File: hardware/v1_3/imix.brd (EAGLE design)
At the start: 87 x 102.5 mm, 154 parts, among them J2_3_5_AND_6 ARDUINO_R3NO_HOLES, U1 BQ2423X, U10 ISL29035, U11 FX0S8700CQ, U12 296-12686-1-ND, U13 SIP32401A, U14 SIP32401A, U15 SIP32401A, U16 SIP32401A, U17 74LVC4066BQ, U18 74LVC4066BQ, U3 TLV3202, U4 LM358, U5 LDO-TPS78233, U6 ATSAM4LCX_100, U8 SI7021, U9 NRF51422, X1 16MHz, X2 16MHz, X3 16MHz

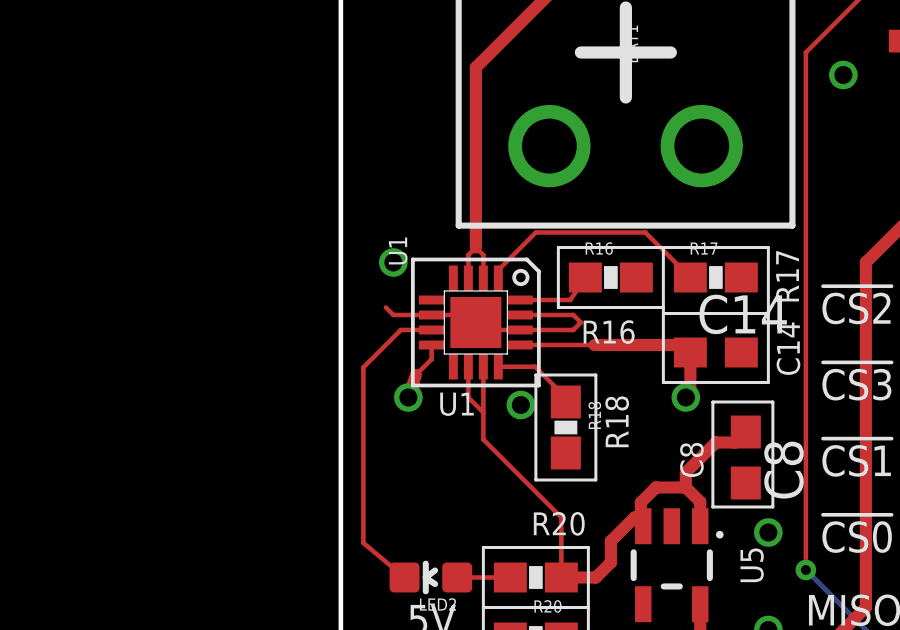
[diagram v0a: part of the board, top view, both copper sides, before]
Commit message: Create PDF
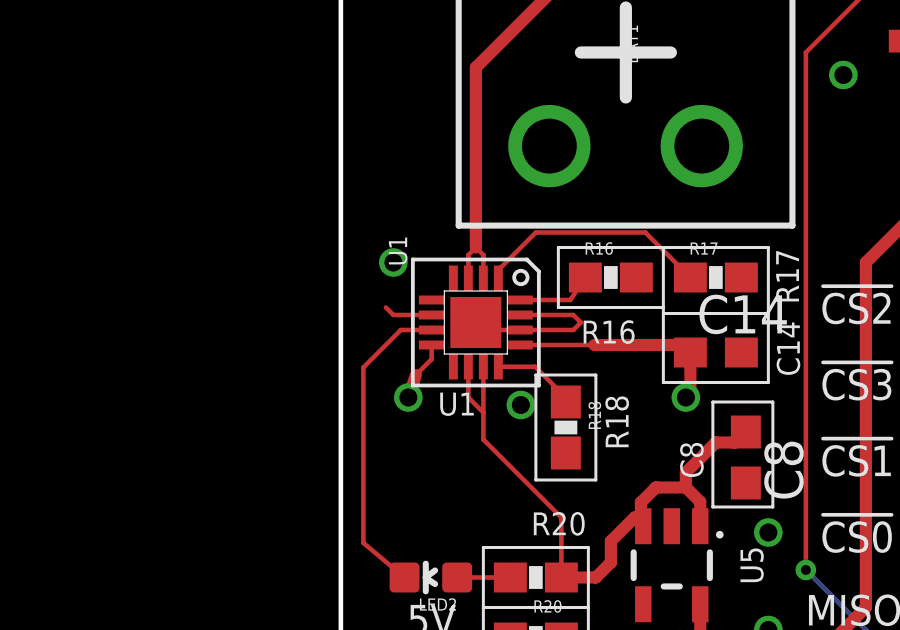
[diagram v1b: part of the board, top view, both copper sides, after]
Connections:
- net GND: no longer U1.6
- net VCC_IN: now also U1.6
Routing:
- net GND: track 215.8 -> 213.0 mm
- net VCC_IN: track 83.9 -> 85.5 mm
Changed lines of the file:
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@@
 <contactref element="R16" pad="2"/>
 <contactref element="U1" pad="4"/>
-<contactref element="U1" pad="6"/>
 <contactref element="U1" pad="5"/>
 <contactref element="U1" pad="14"/>
@@
 <wire x1="50.747" y1="69.824" x2="50.747" y2="67.247" width="0.1524" layer="1"/>
 <wire x1="50.747" y1="67.247" x2="50.5355" y2="67.0355" width="0.1524" layer="1"/>
-<wire x1="3.025" y1="53.25" x2="4.25" y2="53.25" width="0.1524" layer="1"/>
 <wire x1="4.25" y1="53.25" x2="4.5" y2="53" width="0.1524" layer="1"/>
 <via x="43" y="17.5" extent="1-16" drill="0.3302"/>
@@
 <wire x1="77.5" y1="-3.6" x2="79.65" y2="-3.6" width="0.1524" layer="1"/>
 <wire x1="3" y1="53.775" x2="3.025" y2="53.75" width="0.1524" layer="1"/>
-<wire x1="3.025" y1="53.25" x2="1.75" y2="53.25" width="0.1524" layer="1"/>
-<wire x1="1.75" y1="53.25" x2="1.5" y2="53.5" width="0.1524" layer="1"/>
 <wire x1="3.025" y1="52.25" x2="3.025" y2="51.775" width="0.1524" layer="1"/>
 <wire x1="3.025" y1="51.775" x2="2.5" y2="51.25" width="0.1524" layer="1"/>
@@
 <wire x1="6" y1="50.25" x2="7.5" y2="48.65" width="0" layer="19" extent="1-1"/>
 <wire x1="5.975" y1="52.75" x2="6" y2="50.25" width="0" layer="19" extent="1-1"/>
-<wire x1="3.025" y1="53.75" x2="3.025" y2="53.25" width="0" layer="19" extent="1-1"/>
-<wire x1="3.025" y1="52.25" x2="3.025" y2="53.25" width="0" layer="19" extent="1-1"/>
-<wire x1="3.75" y1="54.475" x2="3.025" y2="53.75" width="0" layer="19" extent="1-1"/>
-<wire x1="1.75" y1="55" x2="1.5" y2="53.5" width="0" layer="19" extent="1-1"/>
+<wire x1="3.75" y1="54.475" x2="4.25" y2="53.25" width="0" layer="19" extent="1-1"/>
+<wire x1="3.025" y1="53.75" x2="3.75" y2="54.475" width="0" layer="19" extent="1-1"/>
+<wire x1="3.025" y1="52.25" x2="3.025" y2="53.75" width="0" layer="19" extent="1-1"/>
+<wire x1="1.75" y1="55" x2="3" y2="53.775" width="0" layer="19" extent="1-1"/>
 <wire x1="9.85" y1="54.5" x2="8" y2="53" width="0" layer="19" extent="1-1"/>
 <wire x1="13.35" y1="54.5" x2="9.85" y2="54.5" width="0" layer="19" extent="1-1"/>
@@
 <wire x1="-27.4" y1="-35.5" x2="-24.65" y2="-36.225" width="0" layer="19" extent="1-1"/>
 <wire x1="-27.65" y1="-36.225" x2="-27.4" y2="-35.5" width="0" layer="19" extent="1-1"/>
-<wire x1="-18.55" y1="-43.15" x2="-24.65" y2="-36.225" width="0" layer="19" extent="1-1"/>
+<wire x1="-18.55" y1="-43.15" x2="-18.65" y2="-36.225" width="0" layer="19" extent="1-1"/>
 <wire x1="-20.1" y1="-43.4" x2="-18.55" y2="-43.15" width="0" layer="19" extent="1-1"/>
 <wire x1="-24.85" y1="-45.55" x2="-20.1" y2="-43.4" width="0" layer="19" extent="1-1"/>
@@
 <wire x1="8.5" y1="24.5" x2="9.505" y2="23.495" width="0.4064" layer="1"/>
 <wire x1="9.505" y1="23.495" x2="9.505" y2="23.06" width="0.4064" layer="1"/>
+<contactref element="U1" pad="6"/>
+<wire x1="3.025" y1="53.25" x2="1.75" y2="53.25" width="0.1524" layer="1"/>
+<wire x1="1.75" y1="53.25" x2="1.5" y2="53.5" width="0.1524" layer="1"/>
+<wire x1="5.975" y1="52.25" x2="3.025" y2="53.25" width="0" layer="19" extent="1-1"/>
 </signal>
 <signal name="N$47">
